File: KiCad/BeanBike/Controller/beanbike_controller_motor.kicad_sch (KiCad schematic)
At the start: 8 parts, among them Q1 PHASE A HIGH, Q2 PHASE B HIGH, Q3 PHASE C HIGH, Q4 PHASE A LOW, Q5 PHASE B LOW, Q6 PHASE C LOW, U2 DRV8308

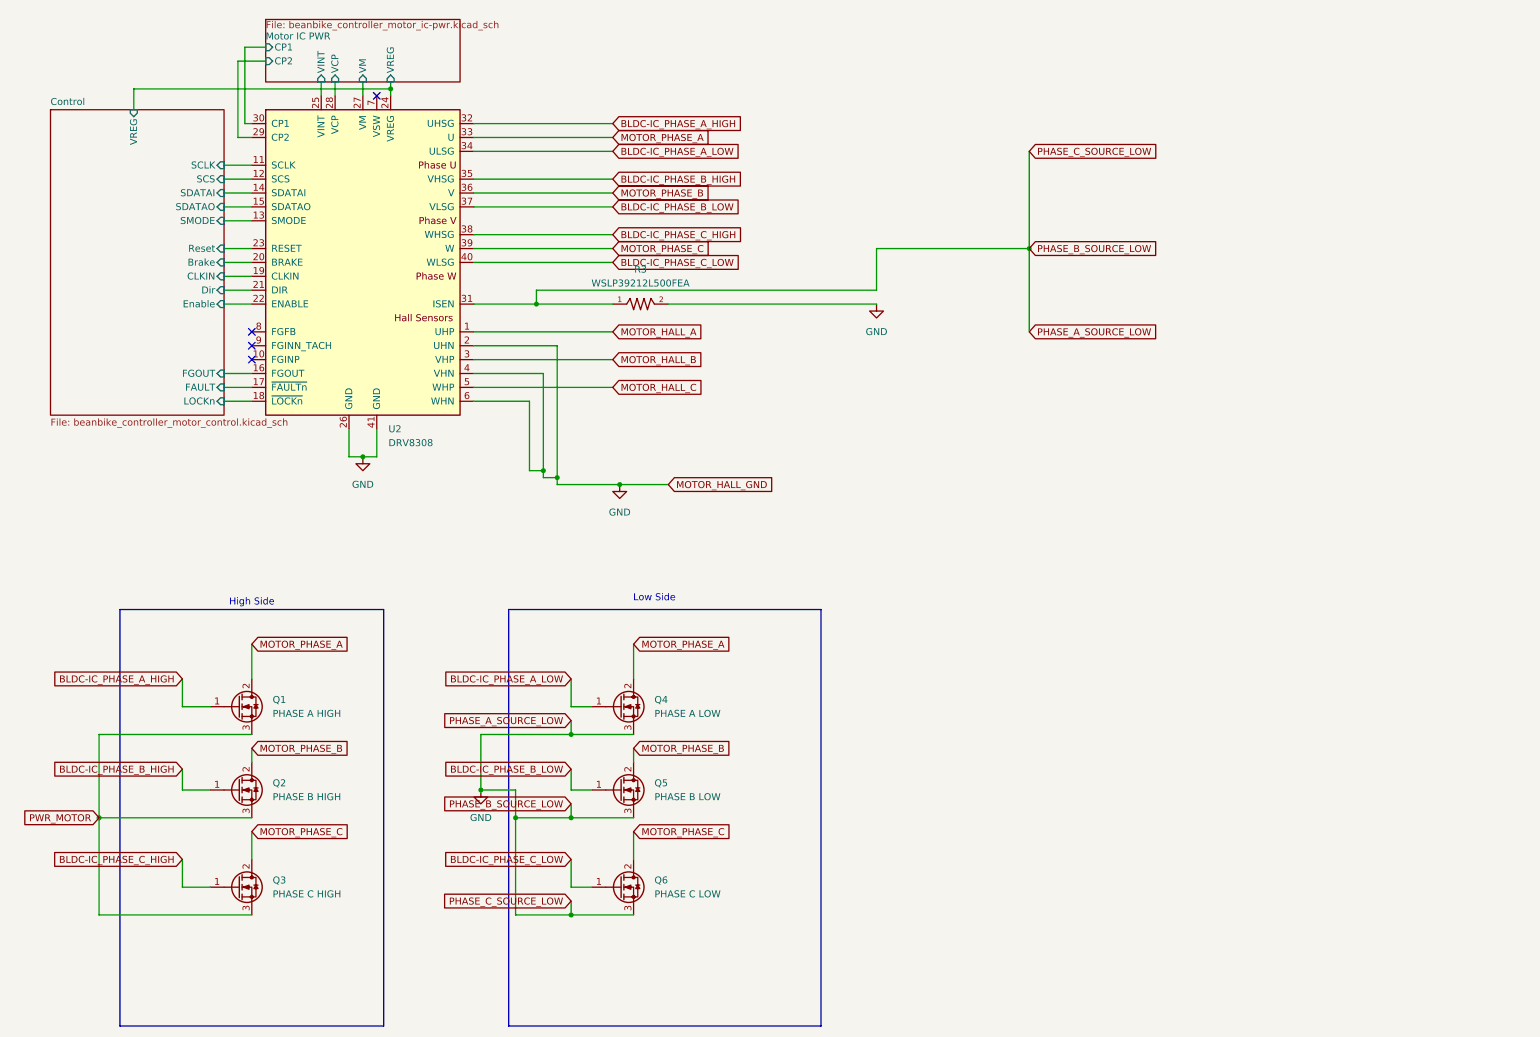
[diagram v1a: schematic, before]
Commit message: PCBv2 Finish
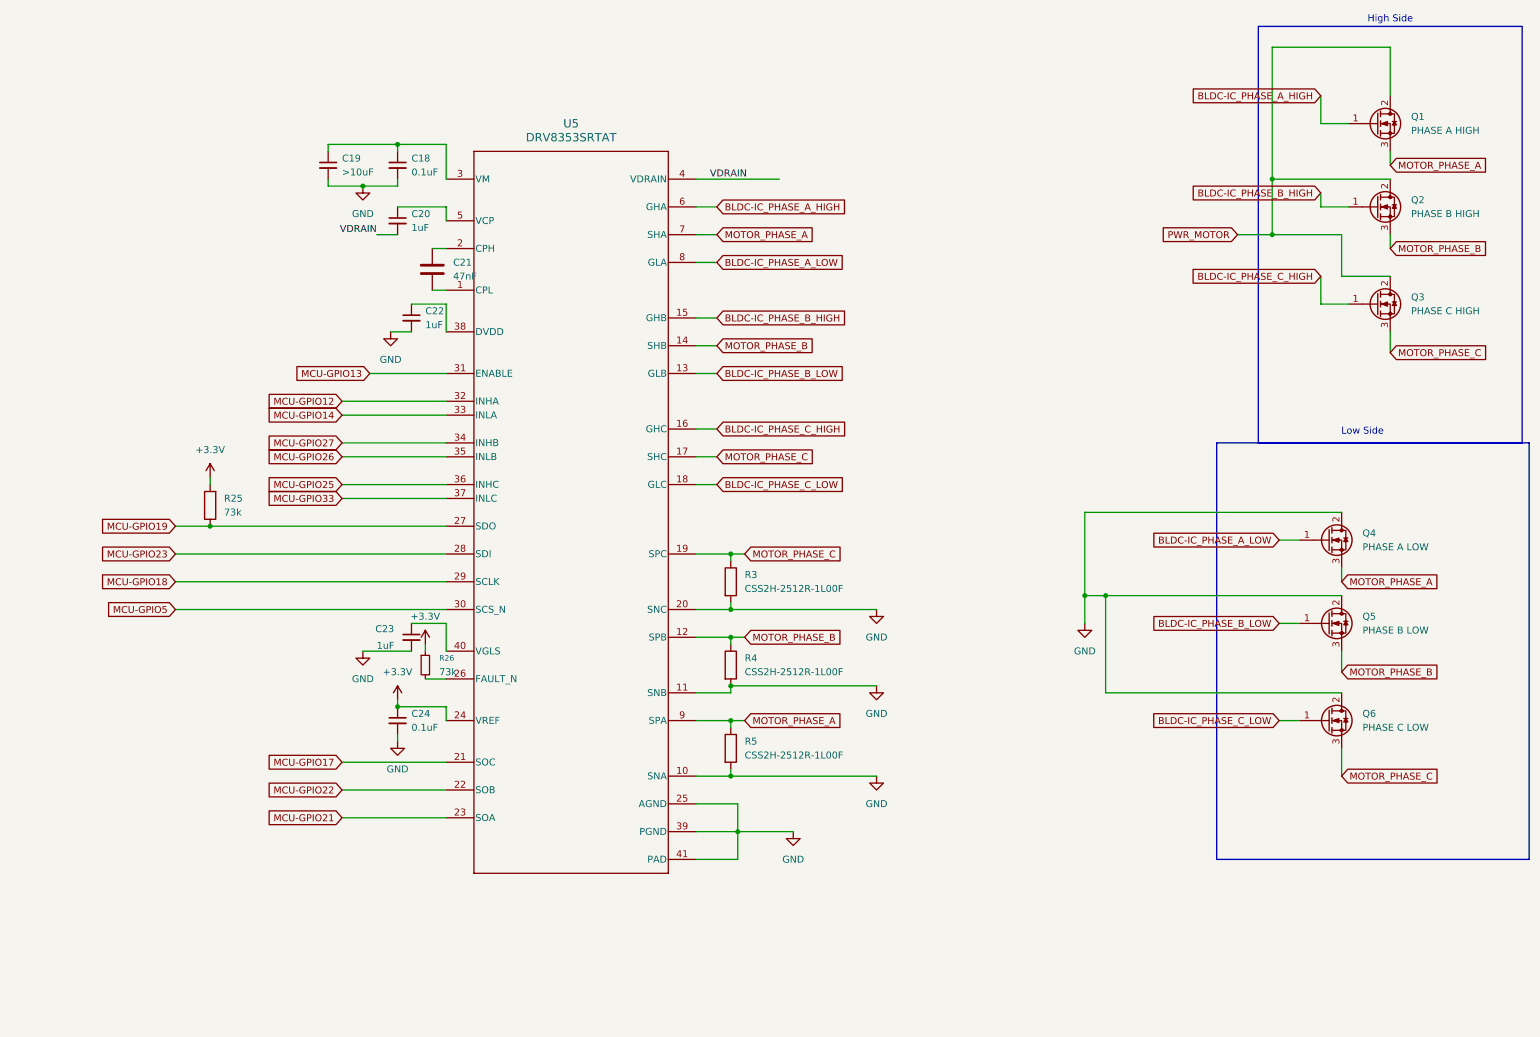
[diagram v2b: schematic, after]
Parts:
- removed R3: WSLP39212L500FEA, WSLP39212L500FEA:RES_WSLP39212L500FEA, symbol WSLP39212L500FEA:WSLP39212L500FEA
- removed U2: DRV8308, Package_DFN_QFN:Texas_RHA0040E_VQFN-40-1EP_6x6mm_P0.5mm_EP3.52x2.62mm, symbol Driver_Motor:DRV8308
- added C18, C24: 0.1uF, Capacitor_SMD:C_0201_0603Metric, symbol Device:C_Small
- added C19: >10uF, Capacitor_SMD:C_0603_1608Metric, symbol Device:C_Small
- added C20, C22, C23: 1uF, Capacitor_SMD:C_0201_0603Metric, symbol Device:C_Small
- added C21: 47nF, Capacitor_SMD:C_0201_0603Metric, symbol Device:C
- added R25: 73k, Resistor_SMD:R_0603_1608Metric, symbol Device:R
- added R26: 73k, Resistor_SMD:R_0603_1608Metric, symbol Device:R_Small
- added R3, R4, R5: CSS2H-2512R-1L00F, Resistor_SMD:R_2512_6332Metric, symbol Device:R
- added U5: DRV8353SRTAT, MOTORIC:RTA0040B, symbol DRV8353:DRV8353SRTAT
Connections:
- net BLDC-IC_PHASE_A_HIGH: now also U5.6 (GHA)
- net BLDC-IC_PHASE_A_LOW: now also U5.8 (GLA)
- net BLDC-IC_PHASE_B_HIGH: now also U5.15 (GHB)
- net BLDC-IC_PHASE_B_LOW: now also U5.13 (GLB)
- net BLDC-IC_PHASE_C_HIGH: now also U5.16 (GHC)
- net BLDC-IC_PHASE_C_LOW: now also U5.18 (GLC)
- net GND: now also Q4.2 (D), Q5.2 (D), Q6.2 (D), C18.2, C19.2, C22.2, C23.2, C24.2, R3.2, R4.2, R5.2, U5.10 (SNA), U5.11 (SNB), U5.20 (SNC), U5.25 (AGND), U5.39 (PGND), U5.41 (PAD); no longer Q4.3 (S), Q5.3 (S), Q6.3 (S)
- net MOTOR_PHASE_A: now also Q1.3 (S), Q4.3 (S), R5.1, U5.7 (SHA), U5.9 (SPA); no longer Q1.2 (D), Q4.2 (D)
- net MOTOR_PHASE_B: now also Q2.3 (S), Q5.3 (S), R4.1, U5.12 (SPB), U5.14 (SHB); no longer Q2.2 (D), Q5.2 (D)
- net MOTOR_PHASE_C: now also Q3.3 (S), Q6.3 (S), R3.1, U5.17 (SHC), U5.19 (SPC); no longer Q3.2 (D), Q6.2 (D)
- net PWR_MOTOR: now also Q1.2 (D), Q2.2 (D), Q3.2 (D); no longer Q1.3 (S), Q2.3 (S), Q3.3 (S)
- new net: C18.1, C19.1, U5.3 (VM)
- new net: C21.2, U5.1 (CPL)
- new net: C21.1, U5.2 (CPH)
- new net: R26.2, U5.26 (FAULT_N)
- new net: C22.1, U5.38 (DVDD)
- new net: C23.1, U5.40 (VGLS)
- new net: C20.1, U5.5 (VCP)
- new net +3.3V: C24.1, R25.2, R26.1, U5.24 (VREF)
- new net MCU-GPIO12: U5.32 (INHA)
- new net MCU-GPIO13: U5.31 (ENABLE)
- new net MCU-GPIO14: U5.33 (INLA)
- new net MCU-GPIO17: U5.21 (SOC)
- new net MCU-GPIO18: U5.29 (SCLK)
- new net MCU-GPIO19: R25.1, U5.27 (SDO)
- new net MCU-GPIO21: U5.23 (SOA)
- new net MCU-GPIO22: U5.22 (SOB)
- new net MCU-GPIO23: U5.28 (SDI)
- new net MCU-GPIO25: U5.36 (INHC)
- new net MCU-GPIO26: U5.35 (INLB)
- new net MCU-GPIO27: U5.34 (INHB)
- new net MCU-GPIO33: U5.37 (INLC)
- new net MCU-GPIO5: U5.30 (SCS_N)
- new net VDRAIN: C20.2, U5.4 (VDRAIN)
- no-connect marks 4 -> 0
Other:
- removed sheet Control
- removed sheet Motor IC PWR
- moved on the sheet: Q1, Q2, Q3, Q4, Q5, Q6
